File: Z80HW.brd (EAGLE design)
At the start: 50.9 x 18.5 mm, 17 parts, among them IC1 MCP1700-33, IC2 PIC32MZ1024EFE064QFN

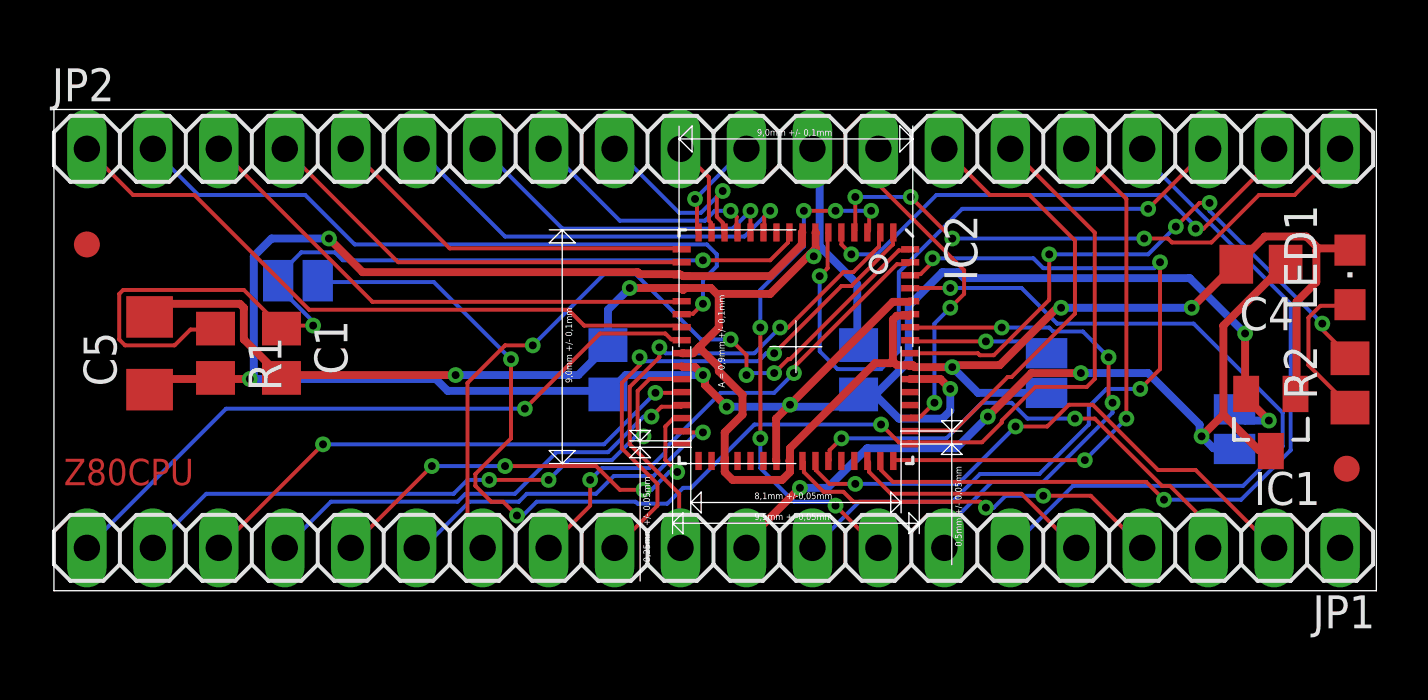
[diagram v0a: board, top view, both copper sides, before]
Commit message: Add files via upload
finito!
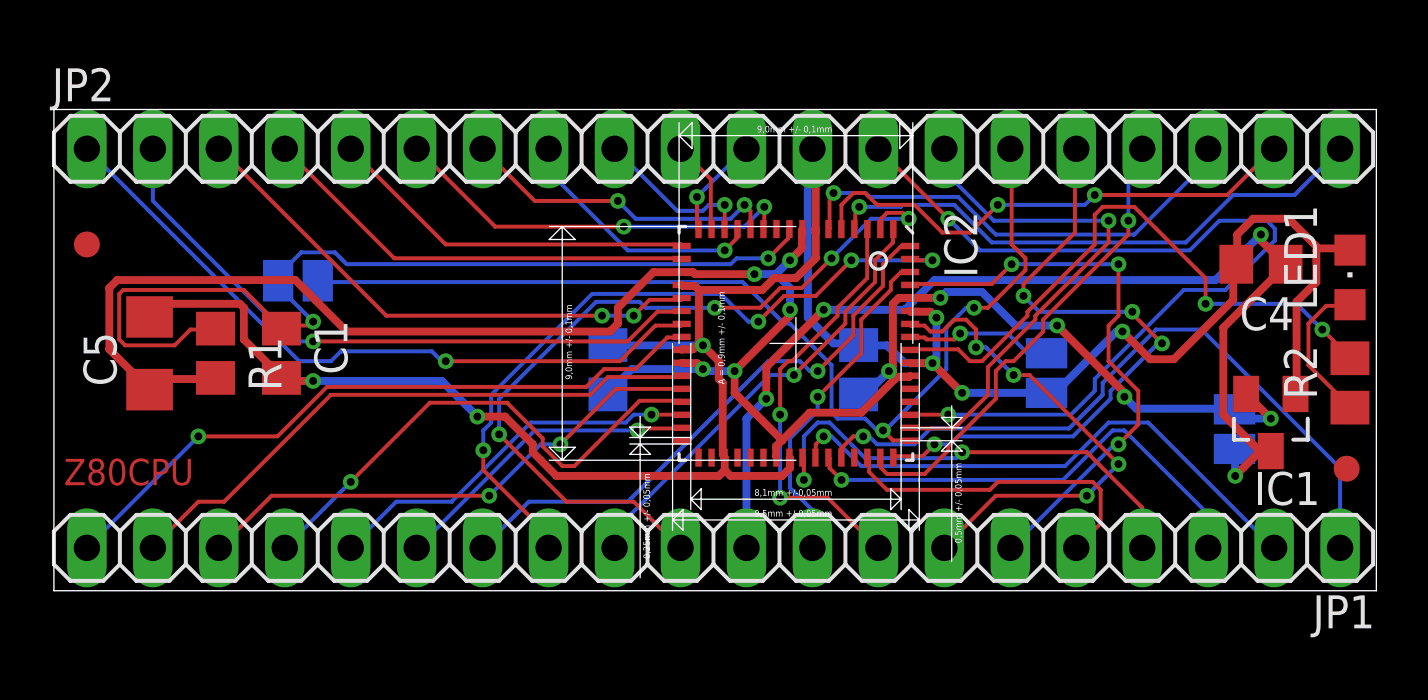
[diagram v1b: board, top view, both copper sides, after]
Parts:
- moved IC2 0.13 mm to (28.6, 9.53)
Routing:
- net IOREQ: track 0.00 -> 27.3 mm, vias 0 -> 1
- net RFSH: track 12.8 -> 35.0 mm
- net D2: track 31.0 -> 13.1 mm, vias 3 -> 1
- net +3V3: track 97.3 -> 81.5 mm, vias 8 -> 10
- net WAIT: track 31.4 -> 18.4 mm
- net RESET: track 51.6 -> 40.3 mm, vias 3 -> 2
- net D6: track 19.9 -> 30.7 mm, vias 2 -> 4
- net D3: track 19.3 -> 28.0 mm, vias 2 -> 4
- net +5V: track 33.6 -> 42.1 mm
- net D1: track 29.7 -> 22.1 mm, vias 1 -> 3
- net BUSAK: track 25.3 -> 18.2 mm, vias 2 -> 1
- net D4: track 29.4 -> 22.5 mm, vias 4 -> 1
- net GND: track 90.8 -> 95.1 mm, vias 6 -> 7
- net BUSRQ: track 20.8 -> 25.0 mm, vias 2 -> 4
- net NMI: track 15.1 -> 18.9 mm
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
